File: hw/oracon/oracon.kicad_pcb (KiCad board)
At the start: 4 copper layers, 81 x 56 mm, 108 parts, among them J2 SIM_Holder, J3 USB_A, J4 Conn_Coaxial, J5 USB_C_Receptacle_USB2.0_16P, Q1 SS8050, Q2 SS8050, Q3 SS8050, Q5 SS8050, SW3 SW_Push, U1 TP5100, U2 AMS1117-3.3, U3 ESP32-S3-MINI-1U, U4 CH343P, U5 TPS61022, U6 MAX3232, U7 SIM7022

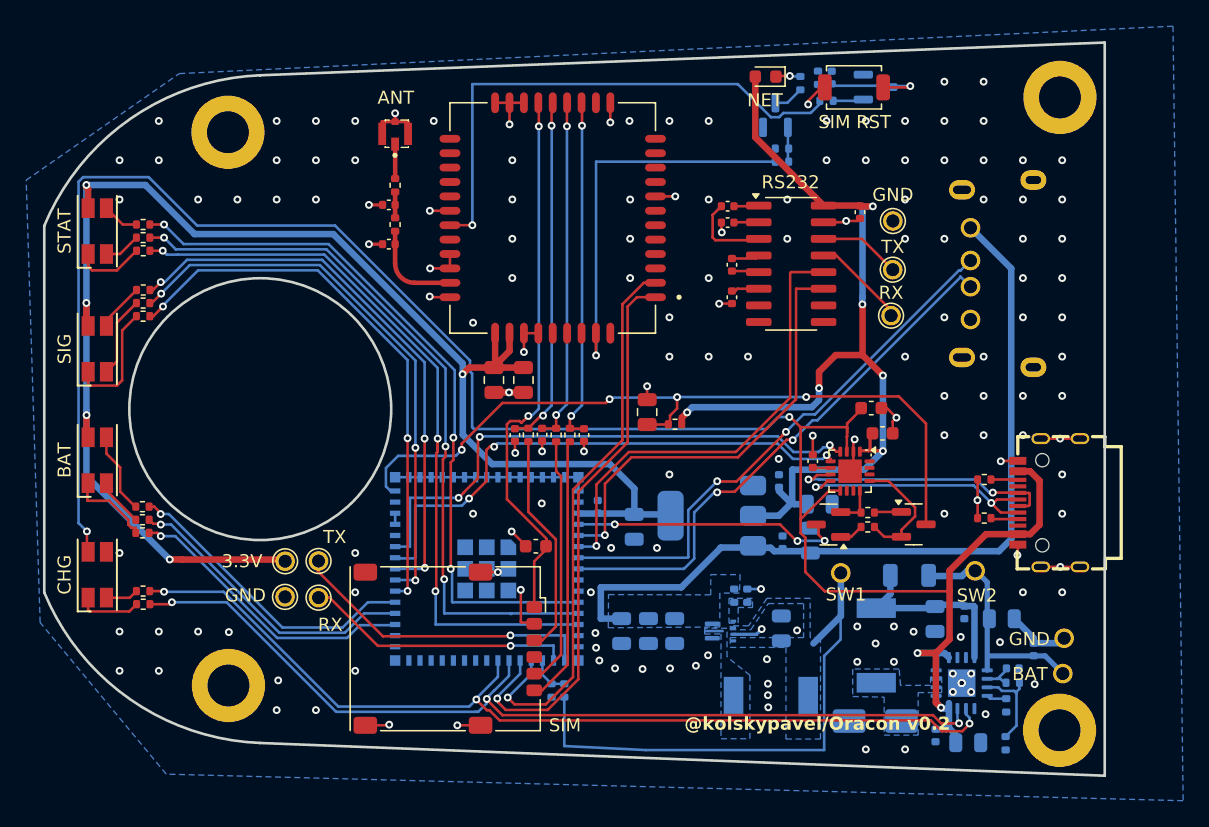
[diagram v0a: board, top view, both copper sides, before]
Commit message: CSQ fix, hw work, cleanup
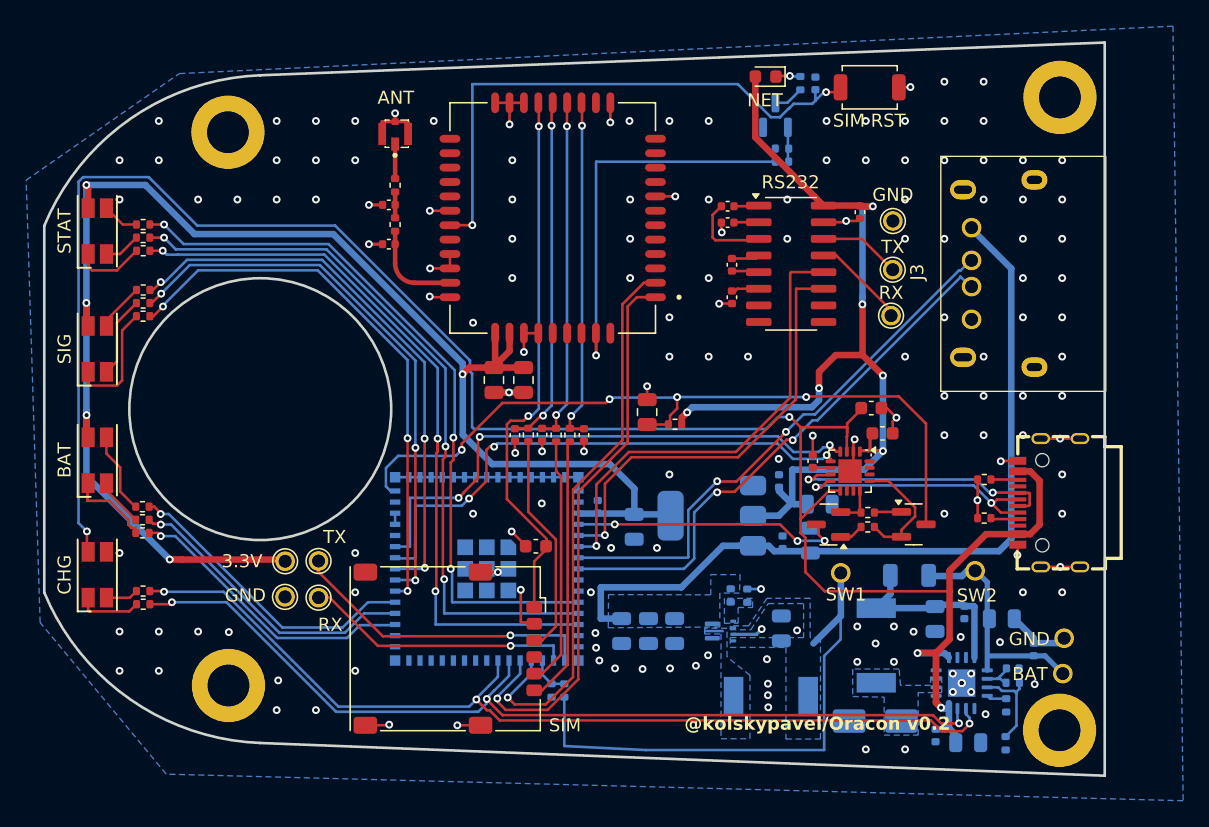
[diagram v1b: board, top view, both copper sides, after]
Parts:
- removed Q5: SS8050, Package_TO_SOT_SMD:SOT-23
- removed R33: 4,7K, Resistor_SMD:R_0402_1005Metric
- removed R34: 47K, Resistor_SMD:R_0402_1005Metric
- C23: value C -> 104
- C27, C28: value C -> DNP
- J3: moved to F.Cu
- R3: value 0R1 -> 120mR
- R31, R32: value R -> 0R
- R4, R6: value x -> DNP
- moved C31 1.33 mm to (22.6, 54.7)
- moved SW3 1.20 mm to (26.8, 55.0), turned to 0 degrees
- moved R13 0.27 mm to (16.1, 93.8)
- moved J3 0.08 mm to (39.3, 69.2), turned to 90 degrees
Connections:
- C31 pad 1: Net-(Q5-C) -> NB_RST
- SW3 pad 1: Net-(Q5-C) -> NB_RST
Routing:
- net Net-(Q5-C): track 8.14 -> 0.00 mm, vias 1 -> 0
- net Net-(Q5-B): track 3.88 -> 0.00 mm
- net NB_RST: track 40.7 -> 43.4 mm, vias 1 -> 2
- net GND: track 88.2 -> 87.1 mm

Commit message: To be checked for production.
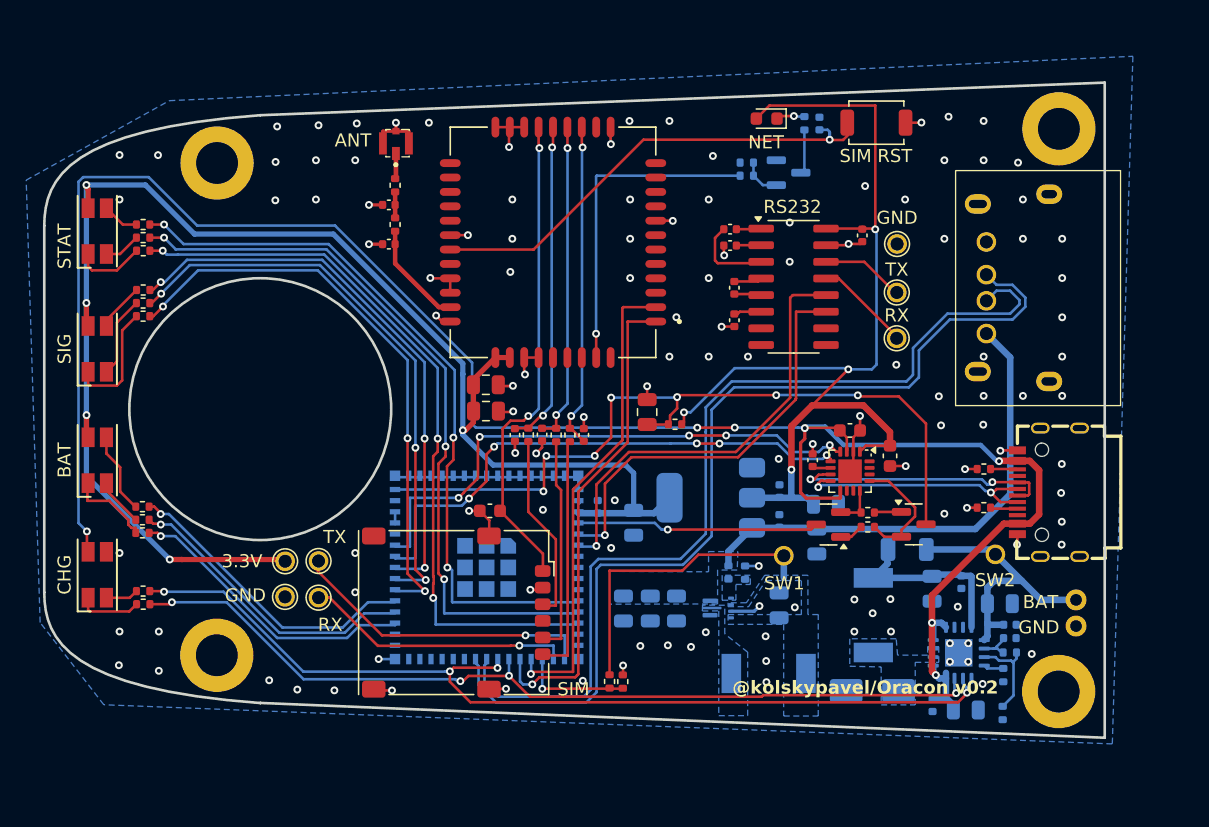
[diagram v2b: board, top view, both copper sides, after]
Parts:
- removed TP1: BATT, TestPoint:TestPoint_Pad_D1.5mm
- removed TP2: GND, TestPoint:TestPoint_Pad_D1.5mm
- added J6: Conn_01x02_MountingPin, kolskypavel:CONN-TH_B2B-PH-K-S, B.Cu at (42.5, 95.2)
- R10, R11: moved to F.Cu
- moved R11 5.49 mm to (7.89, 100.4), turned to -90 degrees
- moved TP4 4.54 mm to (20.2, 90.8)
- moved Q3 4.52 mm to (20.6, 61.5), turned to 0 degrees
- moved C23 4.43 mm to (-2.26, 87.4)
- moved C36 3.72 mm to (-2.56, 79.8), turned to 0 degrees
- moved R10 3.53 mm to (6.88, 100.4), turned to 90 degrees
- moved D6 3.21 mm to (18.9, 57.4)
- moved C31 3.08 mm to (22.9, 57.8)
- moved R27 3.08 mm to (21.8, 57.8)
- moved H4 2.96 mm to (41.2, 101.2)
- moved R12 2.89 mm to (17.4, 60.8)
- moved R26 2.89 mm to (17.4, 61.8)
- moved J2 2.83 mm to (-5.03, 95.1)
- moved SW3 2.75 mm to (27.3, 57.7)
- moved C4 2.62 mm to (37.5, 96.1), turned to 0 degrees
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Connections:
- U3 pad 23: unconnected-(U3-IO19-Pad23) -> USB_SI_N
- U3 pad 24: unconnected-(U3-IO20-Pad24) -> USB_SI_P
- U3 pad 7: USB_SI_N -> unconnected-(U3-IO3-Pad7)
- U3 pad 8: USB_SI_P -> unconnected-(U3-IO4-Pad8)
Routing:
- net USB_SI_P: track 41.6 -> 73.6 mm, vias 2 -> 0
- net USB_SI_N: track 41.5 -> 71.3 mm, vias 2 -> 0
- net +5V: track 62.5 -> 37.5 mm
- net VCC: track 41.0 -> 23.5 mm
- net GND: track 87.1 -> 72.3 mm, vias 161 -> 126
- net VBUS: track 165.0 -> 155.8 mm, vias 4 -> 7
- net NBIOT_RX: track 44.0 -> 37.2 mm
- net NBIOT_TX: track 42.9 -> 36.4 mm
- net NB_RST: track 43.4 -> 37.0 mm, vias 2 -> 1
- net NETLIGHT: track 30.2 -> 24.9 mm
- net ADC_BATT: track 3.26 -> 8.30 mm, vias 0 -> 1
- net SIM_VDD: track 41.9 -> 37.4 mm
- net CHG_STAT: track 71.6 -> 67.4 mm, vias 3 -> 4
- net +3.3V: track 190.5 -> 194.6 mm, vias 11 -> 9
- net +BATT: track 18.2 -> 21.3 mm
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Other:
- board size 81 x 56 mm -> 81 x 50 mm
